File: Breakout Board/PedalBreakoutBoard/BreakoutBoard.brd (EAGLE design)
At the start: 100 x 80 mm, 40 parts, among them U1 ES_DAISY_SEED_REV4

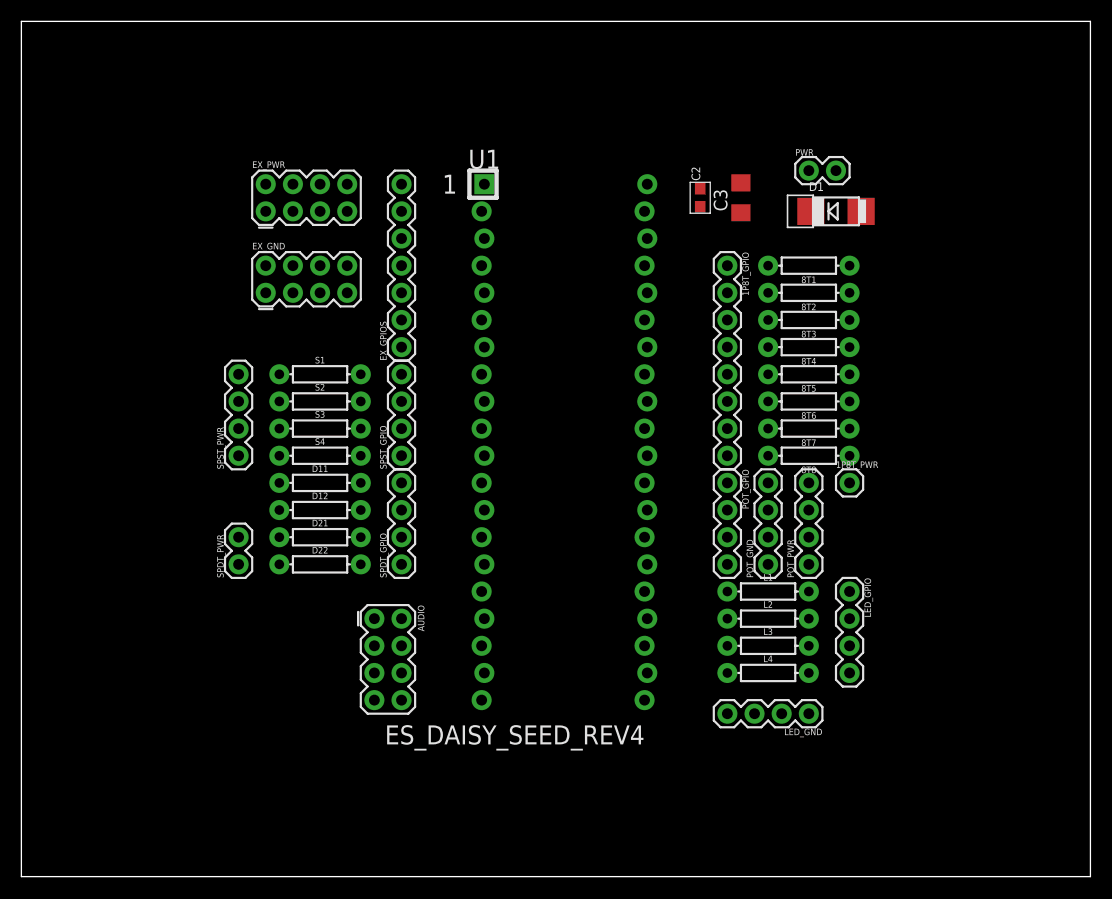
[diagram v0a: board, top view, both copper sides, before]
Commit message: DP-16 - Board layout REV-B
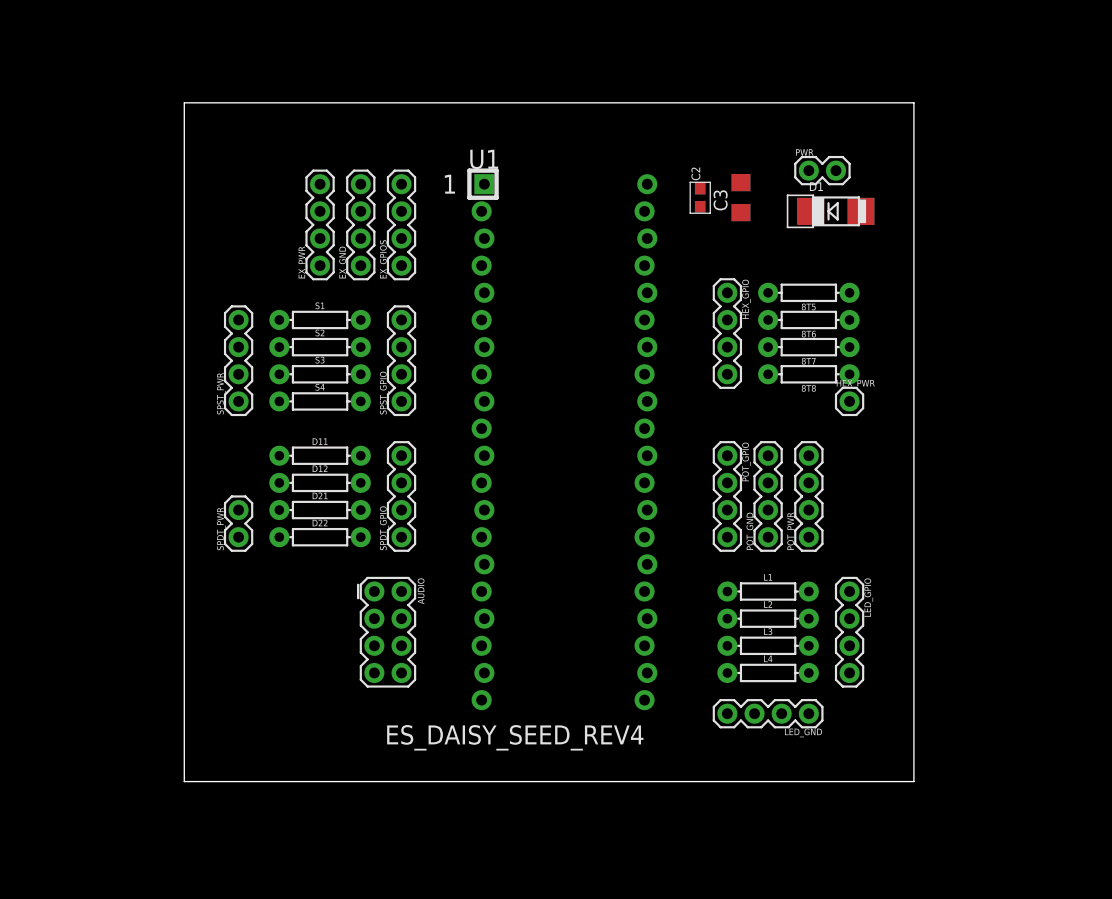
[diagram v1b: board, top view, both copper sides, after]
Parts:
- removed 1P8T_GPIO: (no value), SparkFun-Connectors:1X08
- removed 1P8T_PWR: (no value), SparkFun-Connectors:1X01
- removed 8T1, 8T2, 8T3, 8T4: 10k, SparkFun-Resistors:AXIAL-0.3
- added HEX_GPIO: (no value), SparkFun-Connectors:1X04
- added HEX_PWR: (no value), SparkFun-Connectors:1X01
- EX_GND, EX_PWR: device SparkFun-Connectors:2X4 -> SparkFun-Connectors:1X04
- EX_GPIOS: device SparkFun-Connectors:1X07 -> SparkFun-Connectors:1X04
- moved 8T7 7.62 mm to (73.7, 49.5)
- moved 8T8 7.62 mm to (73.7, 47.0)
- moved 8T5 7.62 mm to (73.7, 54.6)
- moved 8T6 7.62 mm to (73.7, 52.1)
- moved EX_GPIOS 7.62 mm to (35.6, 57.1)
- moved EX_PWR 6.48 mm to (27.9, 57.1), turned to 90 degrees
- moved EX_GND 5.24 mm to (31.8, 57.1), turned to 90 degrees
- moved S3 5.08 mm to (27.9, 47.0)
- moved S4 5.08 mm to (27.9, 44.5)
- moved SPST_GPIO 5.08 mm to (35.6, 44.5)
- moved SPST_PWR 5.08 mm to (20.3, 44.5)
- moved S1 5.08 mm to (27.9, 52.1)
- moved S2 5.08 mm to (27.9, 49.5)
- moved AUDIO 2.54 mm to (34.3, 22.9)
- moved D11 2.54 mm to (27.9, 39.4)
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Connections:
- removed net 1P8T_1: 1P8T_GPIO.1, 8T1.P$2, U1.37
- removed net 1P8T_2: 1P8T_GPIO.2, 8T2.P$2, U1.36
- removed net 1P8T_3: 1P8T_GPIO.3, 8T3.P$2, U1.35
- removed net 1P8T_4: 1P8T_GPIO.4, 8T4.P$2, U1.34
- removed net 1P8T_5: 1P8T_GPIO.5, 8T5.P$2, U1.33
- removed net 1P8T_6: 1P8T_GPIO.6, 8T6.P$2, U1.32
- removed net 1P8T_7: 1P8T_GPIO.7, 8T7.P$2, U1.31
- removed net 1P8T_8: 1P8T_GPIO.8, 8T8.P$2, U1.30
- removed net GPIO5: EX_GPIOS.3, U1.5
- removed net GPIO6: EX_GPIOS.2, U1.6
- removed net GPIO7: EX_GPIOS.1, U1.7
- new net HEX_1: 8T5.P$2, HEX_GPIO.1, U1.36
- new net HEX_2: 8T6.P$2, HEX_GPIO.2, U1.35
- new net HEX_3: 8T7.P$2, HEX_GPIO.3, U1.34
- new net HEX_4: 8T8.P$2, HEX_GPIO.4, U1.33
- net +3V3_A: now also HEX_PWR.1; no longer 1P8T_PWR.1, EX_PWR.5, EX_PWR.6, EX_PWR.7, EX_PWR.8
- net GND: no longer 8T1.P$1, 8T2.P$1, 8T3.P$1, 8T4.P$1, EX_GND.5, EX_GND.6, EX_GND.7, EX_GND.8
- net GPIO1: now also EX_GPIOS.4; no longer EX_GPIOS.7
- net GPIO2: now also EX_GPIOS.3; no longer EX_GPIOS.6
- net GPIO3: now also EX_GPIOS.2; no longer EX_GPIOS.5
- net GPIO4: now also EX_GPIOS.1; no longer EX_GPIOS.4
- net POT1: now also U1.30; no longer U1.29
- net POT2: now also U1.29; no longer U1.28
- net POT3: now also U1.28; no longer U1.27
- net POT4: now also U1.27; no longer U1.26
- net SPDT1_1: now also U1.11; no longer U1.12
- net SPDT1_2: now also U1.12; no longer U1.13
- net SPDT2_1: now also U1.13; no longer U1.14
- net SPDT2_2: now also U1.14; no longer U1.15
- net SPST1: now also U1.6; no longer U1.8
- net SPST2: now also U1.7; no longer U1.9
- net SPST3: now also U1.8; no longer U1.10
- net SPST4: now also U1.9; no longer U1.11
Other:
- board size 100 x 80 mm -> 68.2 x 63.5 mm

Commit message: DP-16 - Initial routing
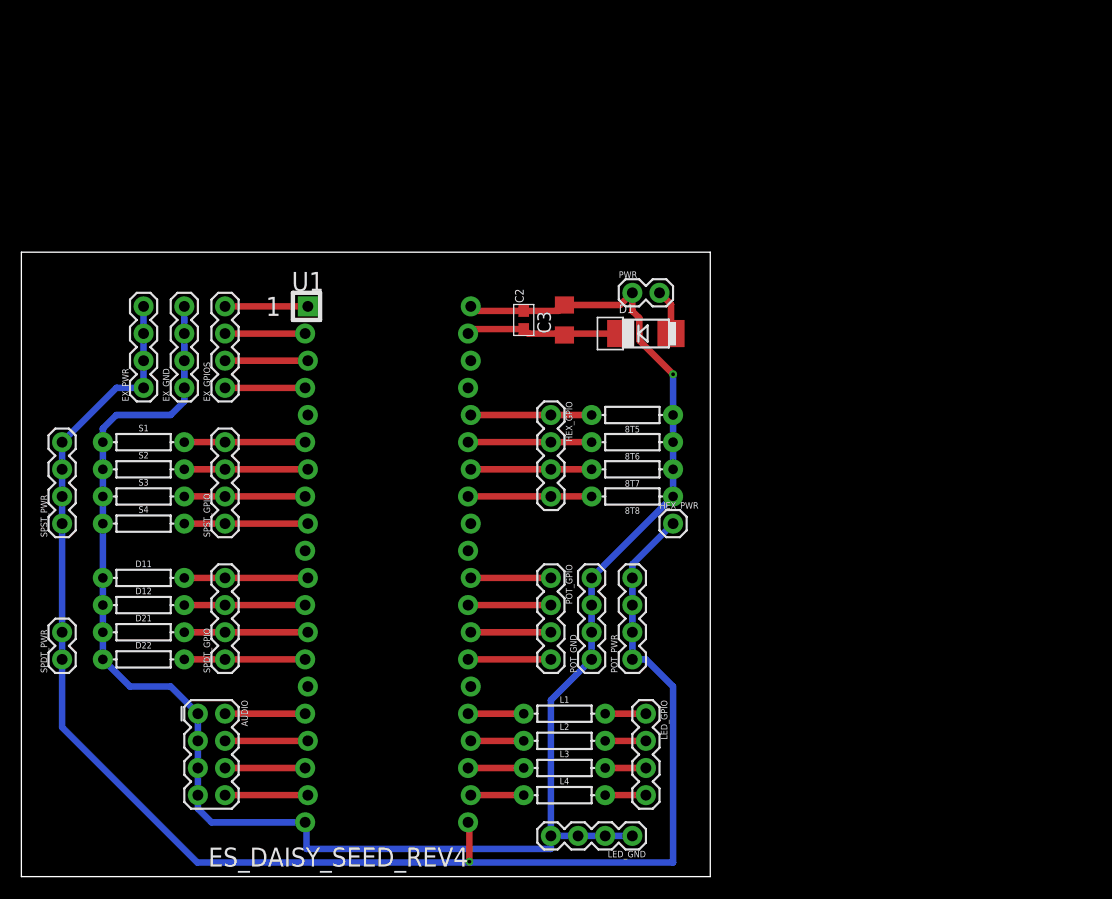
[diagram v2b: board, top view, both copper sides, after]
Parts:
- moved L1 22.2 mm to (50.8, 15.2)
- moved L2 22.2 mm to (50.8, 12.7)
- moved L3 22.2 mm to (50.8, 10.2)
- moved L4 22.2 mm to (50.8, 7.62)
- moved LED_GPIO 22.2 mm to (58.4, 15.2)
- moved D1 21.1 mm to (58.4, 50.8)
- moved C3 20.1 mm to (50.8, 52.1)
- moved D12 20.1 mm to (11.4, 25.4)
- moved D21 20.1 mm to (11.4, 22.9)
- moved D22 20.1 mm to (11.4, 20.3)
- moved EX_GPIOS 20.1 mm to (19.1, 45.7)
- moved EX_PWR 20.1 mm to (11.4, 45.7)
- moved HEX_GPIO 20.1 mm to (49.5, 43.2)
- moved POT_GPIO 20.1 mm to (49.5, 27.9)
- moved PWR 20.1 mm to (57.1, 54.6)
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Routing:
- net GND: track 0.00 -> 176.9 mm, vias 0 -> 1
- net +3V3_A: track 0.00 -> 146.0 mm, vias 0 -> 1
- net +9V_IN: track 0.00 -> 14.8 mm
- net HEX_4: track 0.00 -> 11.6 mm
- net HEX_2: track 0.00 -> 11.6 mm
- net SPST4: track 0.00 -> 11.6 mm
- net SPST2: track 0.00 -> 11.6 mm
- net SPDT2_1: track 0.00 -> 11.6 mm
- net SPDT1_1: track 0.00 -> 11.6 mm
- net HEX_3: track 0.00 -> 11.3 mm
- net HEX_1: track 0.00 -> 11.3 mm
- net SPST3: track 0.00 -> 11.3 mm
- net SPST1: track 0.00 -> 11.3 mm
- net SPDT2_2: track 0.00 -> 11.3 mm
- net SPDT1_2: track 0.00 -> 11.3 mm
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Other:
- board size 68.2 x 63.5 mm -> 64.4 x 58.4 mm
